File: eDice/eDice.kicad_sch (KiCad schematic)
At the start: 25 parts, among them Q1 PMOS, Q2 PN2222A, Q3 PN2222A, SW1 SW_Push, U1 NE555P, U10 4511, U11 SM420561N, U12 4029, U2 4029, U3 4511, U4 SM420561N

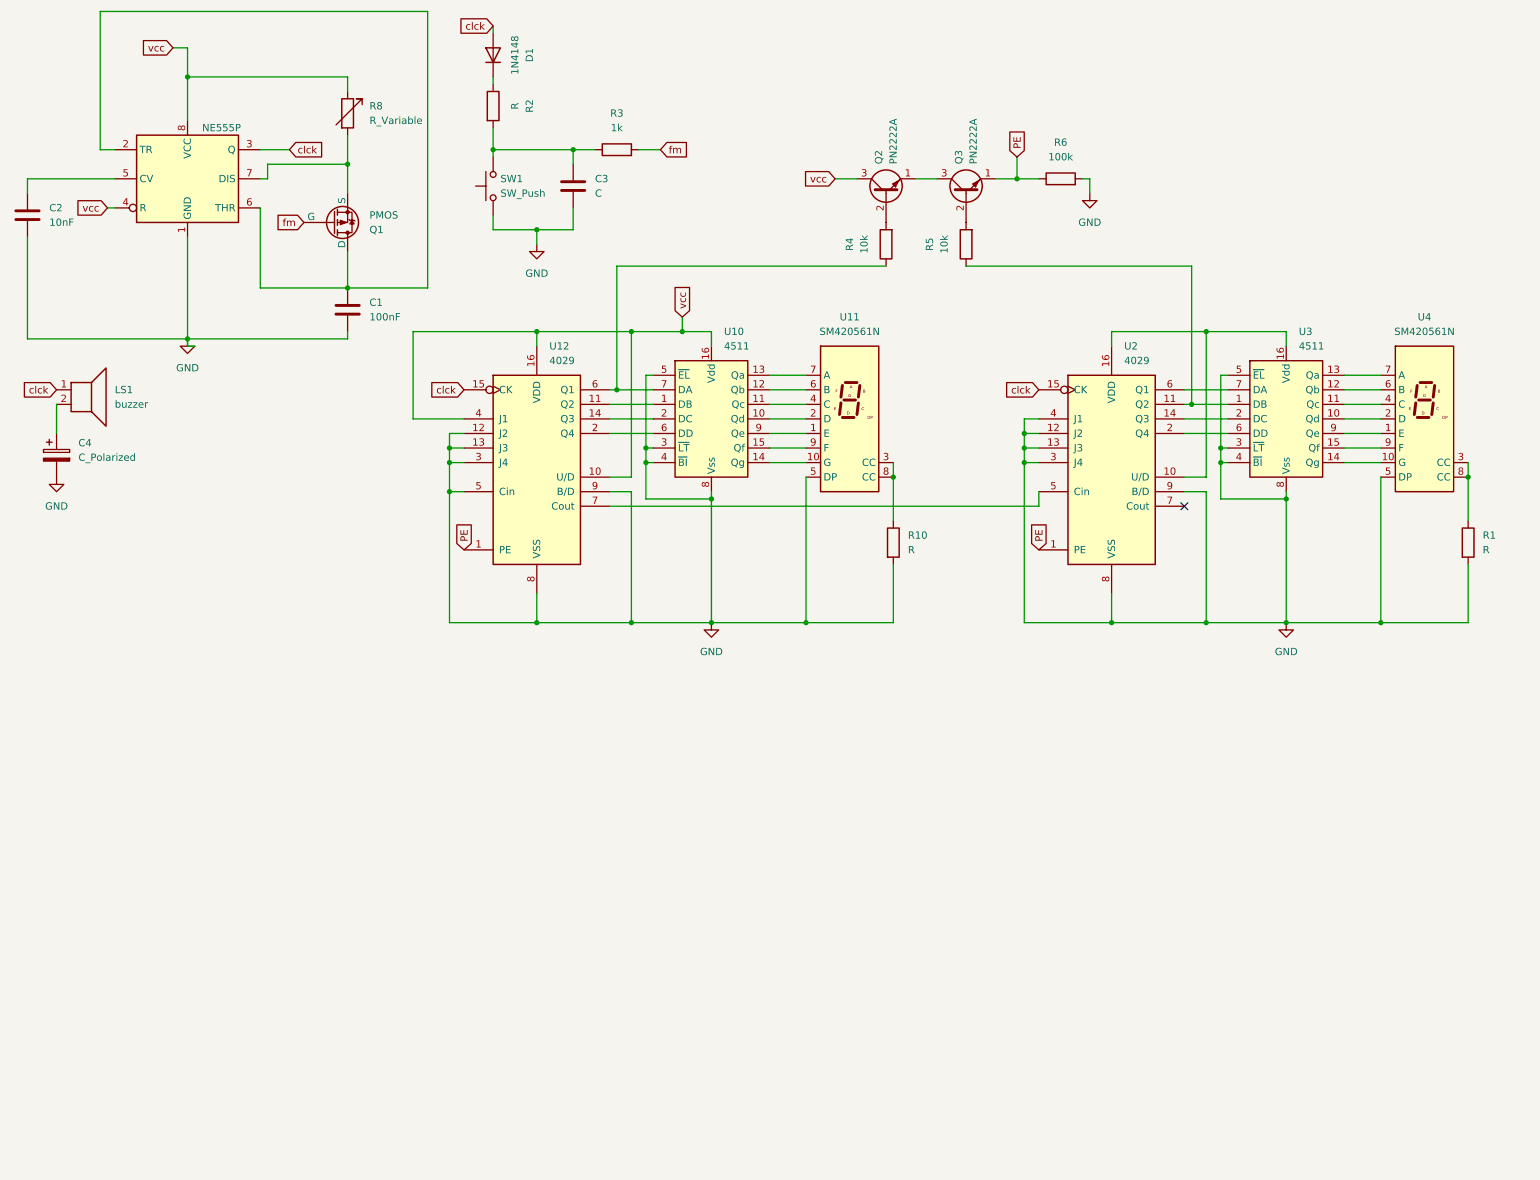
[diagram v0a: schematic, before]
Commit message: update: d6/20
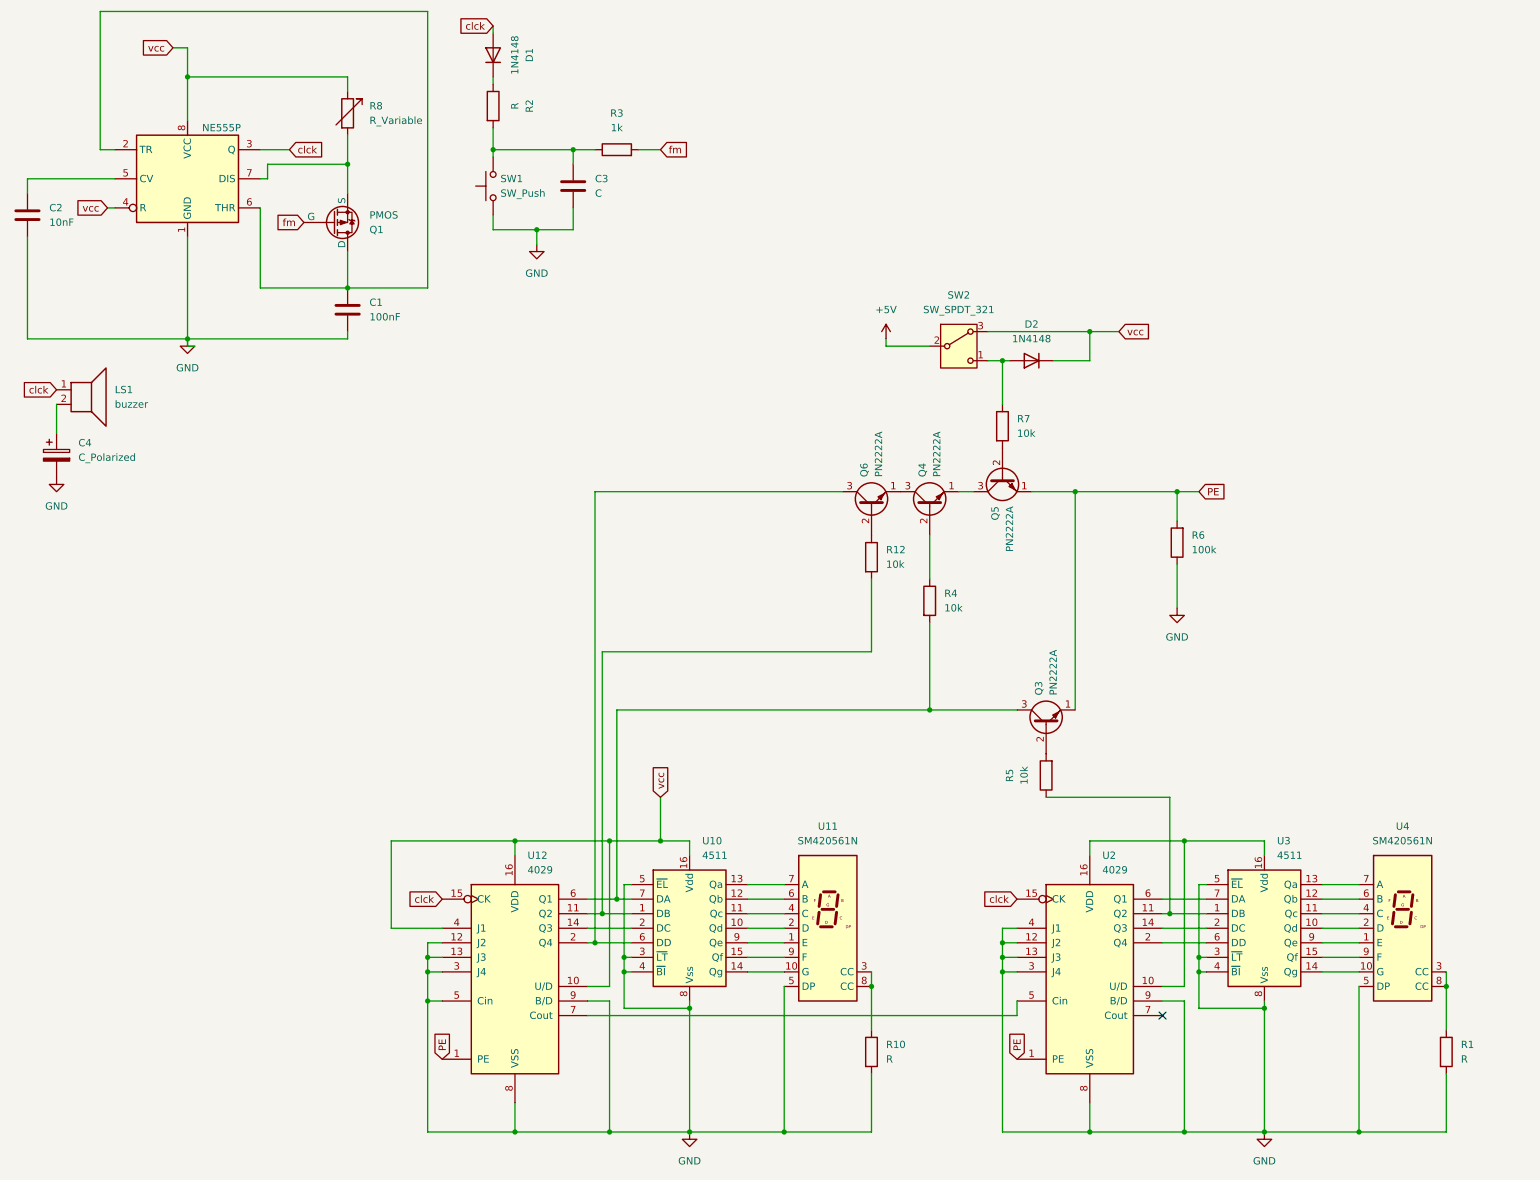
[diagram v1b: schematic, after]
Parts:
- removed Q2: PN2222A, Package_TO_SOT_THT:TO-92_Inline, symbol Transistor_BJT:PN2222A
- added D2: 1N4148, Diode_THT:D_DO-35_SOD27_P7.62mm_Horizontal, symbol Diode:1N4148
- added Q4, Q5, Q6: PN2222A, Package_TO_SOT_THT:TO-92_Inline, symbol Transistor_BJT:PN2222A
- added R12, R7: 10k, Resistor_THT:R_Axial_DIN0204_L3.6mm_D1.6mm_P5.08mm_Horizontal, symbol Device:R
- added SW2: SW_SPDT_321, symbol Switch:SW_SPDT_321
- R6: footprint Resistor_THT:R_Axial_DIN0204_L3.6mm_D1.6mm_P5.08mm_Horizontal -> (none)
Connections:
- net GND: now also R6.1; no longer R6.2
- net PE: now also R6.2, Q5.1 (E); no longer R6.1
- net vcc: now also D2.1 (K), SW2.3 (A)
- net at U10.7 (DA), U12.6 (Q1): now also Q3.3 (C), R4.2; no longer R4.1
- net at U10.1 (DB), U12.11 (Q2): now also R12.2
- net at U10.6 (DD), U12.2 (Q4): now also Q6.3 (C)
- new net: D2.2 (A), R7.1, SW2.1 (C)
- new net: Q5.2 (B), R7.2
- new net: Q4.1 (E), Q5.3 (C)
- new net: Q6.2 (B), R12.1
- new net: Q4.2 (B), R4.1
- new net: Q4.3 (C), Q6.1 (E)
- new net +5V: SW2.2 (B)
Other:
- moved on the sheet: Q3, R1, R10, R5, U10, U11, U12, U2, U3, U4

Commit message: edice
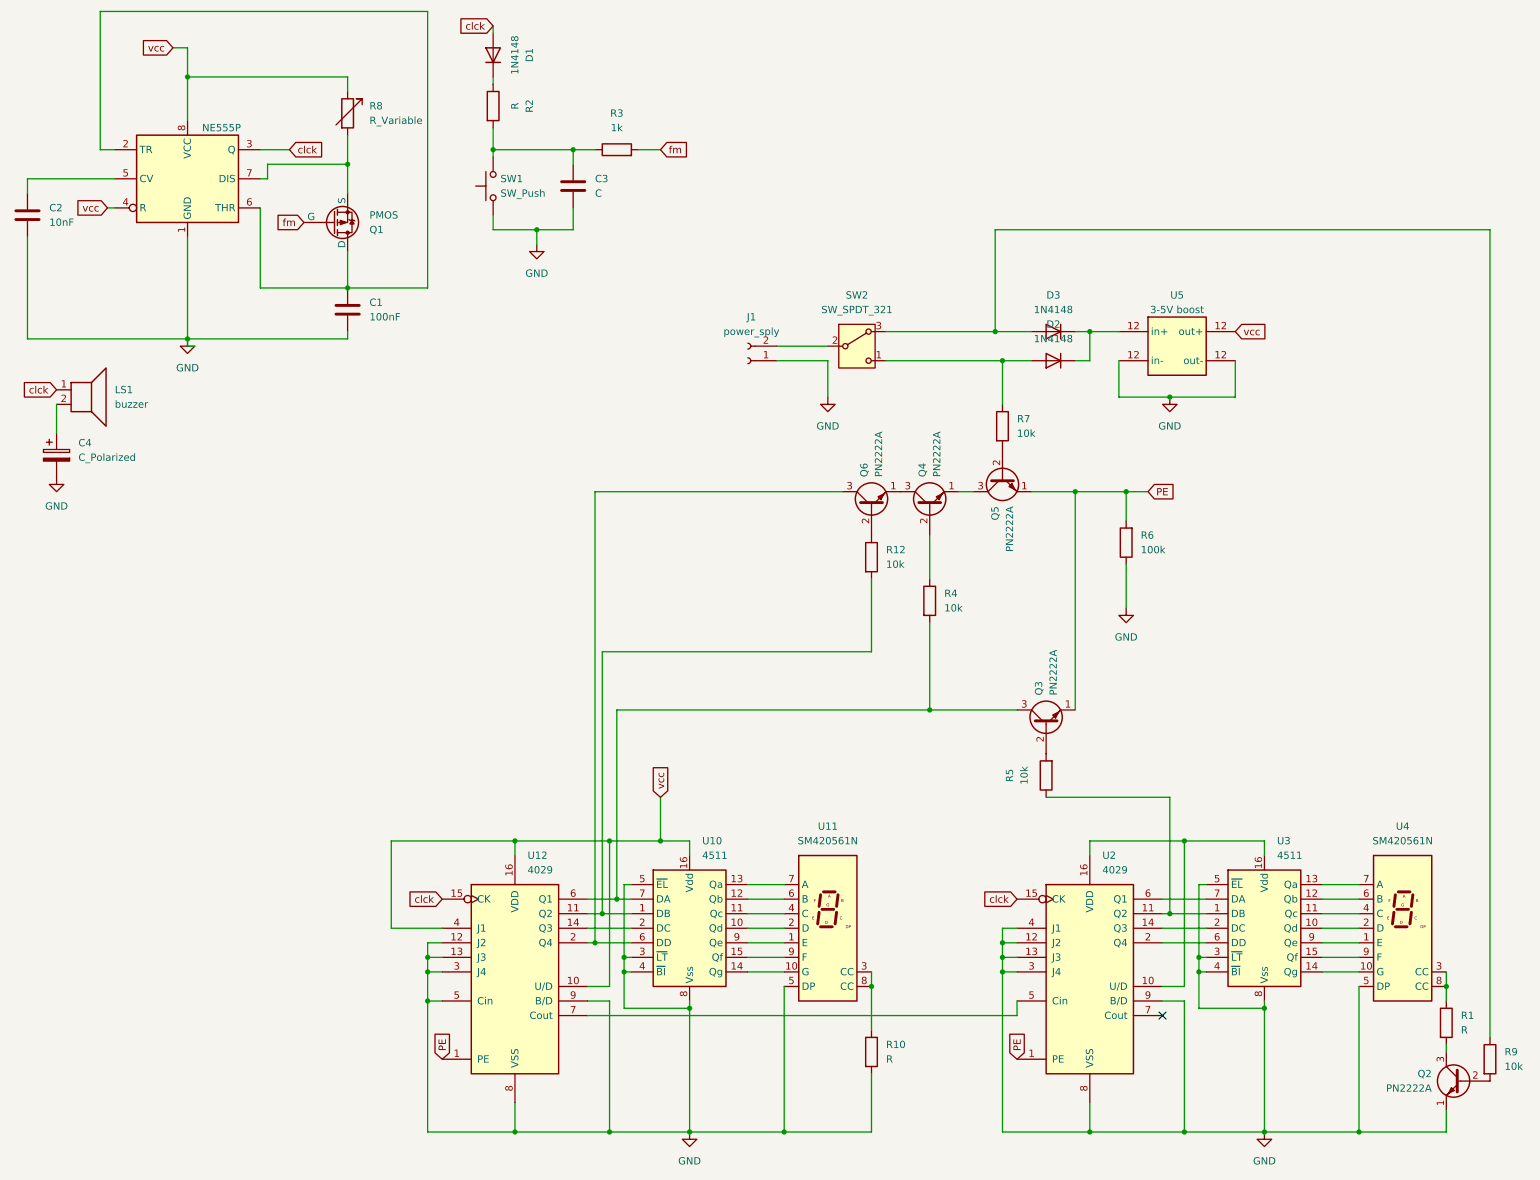
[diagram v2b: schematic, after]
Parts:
- added D3: 1N4148, Diode_THT:D_DO-35_SOD27_P7.62mm_Horizontal, symbol Diode:1N4148
- added J1: power_sply, symbol Connector:Conn_01x02_Socket
- added Q2: PN2222A, Package_TO_SOT_THT:TO-92_Inline, symbol Transistor_BJT:PN2222A
- added R9: 10k, Resistor_THT:R_Axial_DIN0204_L3.6mm_D1.6mm_P5.08mm_Horizontal, symbol Device:R
- added U5: 3-5V boost, symbol eDiceLib:3-5v_boost
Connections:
- net GND: now also J1.1 (Pin_1), Q2.1 (E), U5.12 (out-); no longer R1.2
- net vcc: now also U5.12 (out-); no longer D2.1 (K), SW2.3 (A)
- net +5V: no longer names the net of SW2.2 (B)
- net +5V: now also J1.2 (Pin_2)
- new net: D3.2 (A), R9.1, SW2.3 (A)
- new net: Q2.2 (B), R9.2
- new net: Q2.3 (C), R1.2
- new net: D2.1 (K), D3.1 (K), U5.12 (out-)
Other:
- moved on the sheet: D2, R1, R6
